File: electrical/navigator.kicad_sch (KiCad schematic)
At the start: 5 parts

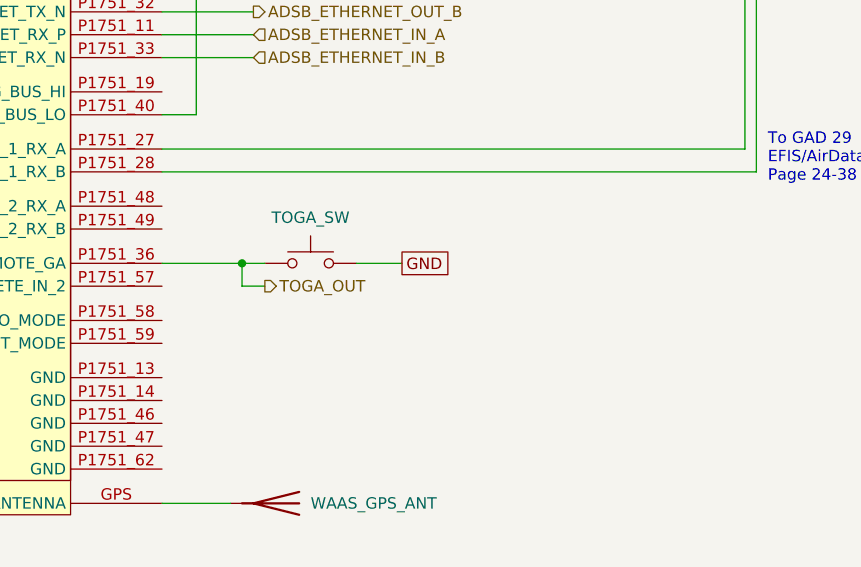
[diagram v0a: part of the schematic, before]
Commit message: Unknown set of changes. Didn't spent time to look
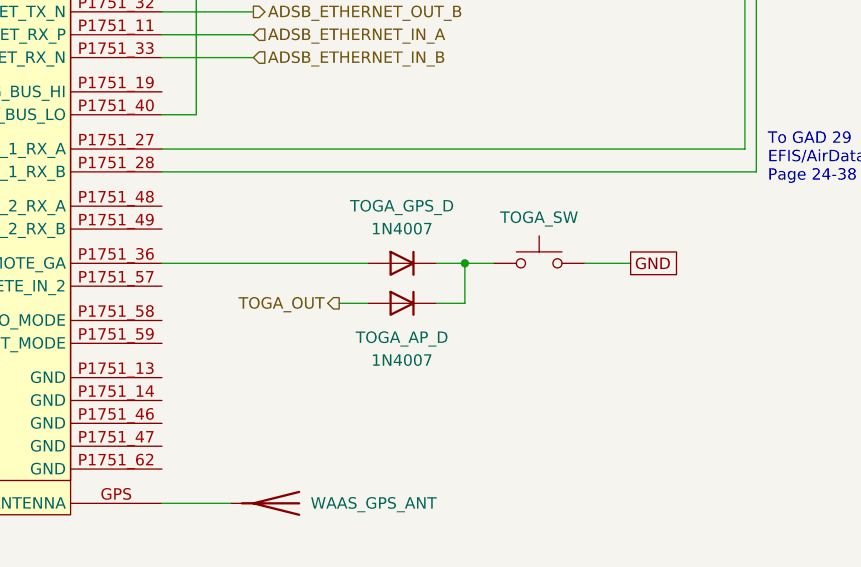
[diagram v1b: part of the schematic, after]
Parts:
- added TOGA_AP_D, TOGA_GPS_D: 1N4007, Diode_THT:D_DO-41_SOD81_P10.16mm_Horizontal, symbol Diode:1N4007
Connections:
- net TOGA_OUT: now also TOGA_AP_D.2 (A); no longer GPS175.P1751_36 (DISCRETE_IN_1/REMOTE_GA), TOGA_SW.1
- new net: TOGA_AP_D.1 (K), TOGA_GPS_D.1 (K), TOGA_SW.1
- new net: GPS175.P1751_36 (DISCRETE_IN_1/REMOTE_GA), TOGA_GPS_D.2 (A)
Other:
- moved on the sheet: TOGA_SW
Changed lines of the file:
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@@
   (title_block
     (date "2024-02-13")
-    (rev "1.0")
+    (rev "1.0.1")
     (comment 1 "w/Breakers")
   )
@@
   (junction (at 152.4 31.75) (diameter 0) (color 0 0 0 0)
   )
+  (junction (at 98.425 172.72) (diameter 0) (color 0 0 0 0)
+  )
   (junction (at 153.67 34.29) (diameter 0) (color 0 0 0 0)
-  )
-  (junction (at 73.66 172.72) (diameter 0) (color 0 0 0 0)
   )
   (junction (at 68.58 26.67) (diameter 0) (color 0 0 0 0)
@@
     (stroke (width 0) (type default))
   )
-  (wire (pts (xy 64.77 172.72) (xy 73.66 172.72))
-    (stroke (width 0) (type default))
-  )
   (wire (pts (xy 64.77 147.32) (xy 74.93 147.32))
     (stroke (width 0) (type default))
   )
+  (wire (pts (xy 64.77 172.72) (xy 87.63 172.72))
+    (stroke (width 0) (type default))
+  )
   (wire (pts (xy 64.77 156.21) (xy 68.58 156.21))
     (stroke (width 0) (type default))
@@
     (stroke (width 0) (type default))
   )
-  (wire (pts (xy 73.66 172.72) (xy 76.2 172.72))
-    (stroke (width 0) (type default))
-  )
   (wire (pts (xy 130.81 162.56) (xy 130.81 53.34))
     (stroke (width 0) (type default))
@@
     (stroke (width 0) (type default))
   )
+  (wire (pts (xy 84.455 177.165) (xy 87.63 177.165))
+    (stroke (width 0) (type default))
+  )
   (wire (pts (xy 129.54 160.02) (xy 129.54 48.26))
     (stroke (width 0) (type default))
   )
+  (wire (pts (xy 95.25 177.165) (xy 98.425 177.165))
+    (stroke (width 0) (type default))
+  )
   (wire (pts (xy 64.77 77.47) (xy 73.66 77.47))
     (stroke (width 0) (type default))
@@
     (stroke (width 0) (type default))
   )
-  (wire (pts (xy 73.66 175.26) (xy 73.66 172.72))
-    (stroke (width 0) (type default))
-  )
   (wire (pts (xy 64.77 24.13) (xy 72.39 24.13))
     (stroke (width 0) (type default))
@@
     (stroke (width 0) (type default))
   )
-  (wire (pts (xy 86.36 172.72) (xy 91.44 172.72))
+  (wire (pts (xy 111.76 172.72) (xy 116.84 172.72))
     (stroke (width 0) (type default))
   )
@@
     (stroke (width 0) (type default))
   )
-  (wire (pts (xy 76.2 175.26) (xy 73.66 175.26))
-    (stroke (width 0) (type default))
-  )
   (wire (pts (xy 64.77 144.78) (xy 74.93 144.78))
     (stroke (width 0) (type default))
@@
     (stroke (width 0) (type default))
   )
+  (wire (pts (xy 98.425 177.165) (xy 98.425 172.72))
+    (stroke (width 0) (type default))
+  )
   (wire (pts (xy 64.77 88.9) (xy 73.66 88.9))
     (stroke (width 0) (type default))
@@
     (stroke (width 0) (type default))
   )
+  (wire (pts (xy 95.25 172.72) (xy 98.425 172.72))
+    (stroke (width 0) (type default))
+  )
   (wire (pts (xy 64.77 26.67) (xy 68.58 26.67))
+    (stroke (width 0) (type default))
+  )
+  (wire (pts (xy 98.425 172.72) (xy 101.6 172.72))
     (stroke (width 0) (type default))
   )
@@
     )
   )
-  (global_label "GND" (shape passive) (at 91.44 172.72 0) (fields_autoplaced)
-    (effects (font (size 1.27 1.27)) (justify left))
-    (property "Intersheetrefs" "${INTERSHEET_REFS}" (at 97.1844 172.72 0)
+  (global_label "GND" (shape passive) (at 116.84 172.72 0) (fields_autoplaced)
+    (effects (font (size 1.27 1.27)) (justify left))
+    (property "Intersheetrefs" "${INTERSHEET_REFS}" (at 122.5844 172.72 0)
       (effects (font (size 1.27 1.27)) (justify left) hide)
     )
@@
     (effects (font (size 1.27 1.27)) (justify right))
   )
-  (hierarchical_label "TOGA_OUT" (shape output) (at 76.2 175.26 0) (fields_autoplaced)
-    (effects (font (size 1.27 1.27)) (justify left))
+  (hierarchical_label "TOGA_OUT" (shape output) (at 84.455 177.165 180) (fields_autoplaced)
+    (effects (font (size 1.27 1.27)) (justify right))
+  )
+  (symbol (lib_id "Diode:1N4007") (at 91.44 177.165 0) (mirror y) (unit 1)
+    (in_bom yes) (on_board yes) (dnp no)
+    (property "Reference" "TOGA_AP_D" (at 91.44 180.975 0)
+      (effects (font (size 1.27 1.27)))
+    )
+    (property "Value" "1N4007" (at 91.44 183.515 0)
+      (effects (font (size 1.27 1.27)))
+    )
+    (property "Footprint" "Diode_THT:D_DO-41_SOD81_P10.16mm_Horizontal" (at 91.44 181.61 0)
+      (effects (font (size 1.27 1.27)) hide)
+    )
+    (property "Datasheet" "http://www.vishay.com/docs/88503/1n4001.pdf" (at 91.44 177.165 0)
+      (effects (font (size 1.27 1.27)) hide)
+    )
+    (property "Sim.Device" "D" (at 91.44 177.165 0)
+      (effects (font (size 1.27 1.27)) hide)
+    )
+    (property "Sim.Pins" "1=K 2=A" (at 91.44 177.165 0)
+      (effects (font (size 1.27 1.27)) hide)
+    )
+    (pin "2")
+    (pin "1")
+    (instances
+      (project "electrical"
+        (path "/e8ec215a-dbe2-4eba-a577-e50a0a128049/a7d1a714-f940-4397-adef-d76b5058aa57"
+          (reference "TOGA_AP_D") (unit 1)
+        )
+      )
+    )
   )
   (symbol (lib_id "flyerx:Garmin_Config") (at 82.55 34.29 0) (mirror y) (unit 1)
@@
         (path "/e8ec215a-dbe2-4eba-a577-e50a0a128049/a7d1a714-f940-4397-adef-d76b5058aa57"
           (reference "GPS175_CONFIG") (unit 1)
+        )
+      )
+    )
+  )
+  (symbol (lib_id "Diode:1N4007") (at 91.44 172.72 0) (mirror y) (unit 1)
+    (in_bom yes) (on_board yes) (dnp no)
+    (property "Reference" "TOGA_GPS_D" (at 91.44 166.37 0)
+      (effects (font (size 1.27 1.27)))
+    )
+    (property "Value" "1N4007" (at 91.44 168.91 0)
+      (effects (font (size 1.27 1.27)))
+    )
+    (property "Footprint" "Diode_THT:D_DO-41_SOD81_P10.16mm_Horizontal" (at 91.44 177.165 0)
+      (effects (font (size 1.27 1.27)) hide)
+    )
+    (property "Datasheet" "http://www.vishay.com/docs/88503/1n4001.pdf" (at 91.44 172.72 0)
+      (effects (font (size 1.27 1.27)) hide)
+    )
+    (property "Sim.Device" "D" (at 91.44 172.72 0)
+      (effects (font (size 1.27 1.27)) hide)
+    )
+    (property "Sim.Pins" "1=K 2=A" (at 91.44 172.72 0)
+      (effects (font (size 1.27 1.27)) hide)
+    )
+    (pin "2")
+    (pin "1")
+    (instances
+      (project "electrical"
+        (path "/e8ec215a-dbe2-4eba-a577-e50a0a128049/a7d1a714-f940-4397-adef-d76b5058aa57"
+          (reference "TOGA_GPS_D") (unit 1)
         )
       )
@@
     )
   )
-  (symbol (lib_id "Switch:SW_Push") (at 81.28 172.72 0) (unit 1)
+  (symbol (lib_id "Switch:SW_Push") (at 106.68 172.72 0) (unit 1)
     (in_bom yes) (on_board yes) (dnp no)
-    (property "Reference" "TOGA_SW" (at 81.28 167.64 0)
-      (effects (font (size 1.27 1.27)))
-    )
-    (property "Value" "SW_Push" (at 81.28 167.64 0)
-      (effects (font (size 1.27 1.27)) hide)
-    )
-    (property "Footprint" "" (at 81.28 167.64 0)
-      (effects (font (size 1.27 1.27)) hide)
-    )
-    (property "Datasheet" "~" (at 81.28 167.64 0)
-      (effects (font (size 1.27 1.27)) hide)
-    )
+    (property "Reference" "TOGA_SW" (at 106.68 167.64 0)
+      (effects (font (size 1.27 1.27)))
+    )
+    (property "Value" "SW_Push" (at 106.68 167.64 0)
+      (effects (font (size 1.27 1.27)) hide)
+    )
+    (property "Footprint" "" (at 106.68 167.64 0)
+      (effects (font (size 1.27 1.27)) hide)
+    )
+    (property "Datasheet" "~" (at 106.68 167.64 0)
+      (effects (font (size 1.27 1.27)) hide)
+    )
